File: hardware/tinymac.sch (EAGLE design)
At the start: 29 parts, among them IC1 LPC1114FN28, J1 ZX62-B-5PA, SW1 TACT_SW, SW2 TACT_SW, SW3 TACT_SW, SW4 TACT_SW, SW5 TACT_SW, T1 TA48M033F

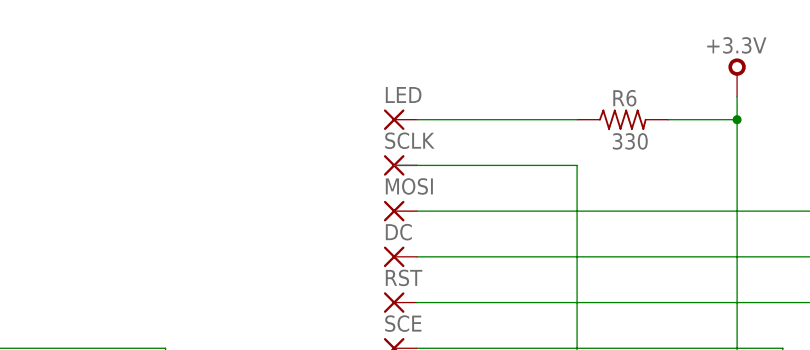
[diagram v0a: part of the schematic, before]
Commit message: change DRU setting to Seeed-2layer-DRU
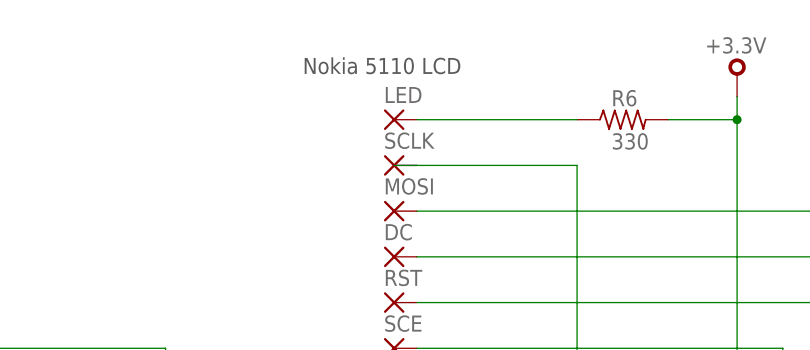
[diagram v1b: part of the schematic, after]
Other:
- note added: "Nokia 5110 LCD"
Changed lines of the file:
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@@
 <sheet>
 <plain>
+<text x="78.74" y="170.18" size="1.778" layer="97">Nokia 5110 LCD</text>
 </plain>
 <instances>
